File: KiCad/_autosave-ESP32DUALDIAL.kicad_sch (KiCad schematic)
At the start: 84 parts, among them J1 SERVICE, J2 Conn_01x04_Male, J3 mode, J5 Conn_01x03_Male, J6 Conn_01x02_Male, J7 Conn_01x02_Male, J8 Conn_01x02_Male, M1 Fan_CPU_4pin, M2 Fan_CPU_4pin, Q1 Q_NMOS_GDS, SW1 Rotary_Encoder_Switch, SW2 Rotary_Encoder_Switch, U1 CR2013-MI2120, U10 Mini560_DC-DC_JW5068A, U2 ESP-WROOM-32, U3 QS-1205CME-3A_MINIDC-DC_12-24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, U4 DHT11, U5 S108T02, U6 S108T02, U7 S108T02, U8 S108T02, U9 TBD62783A

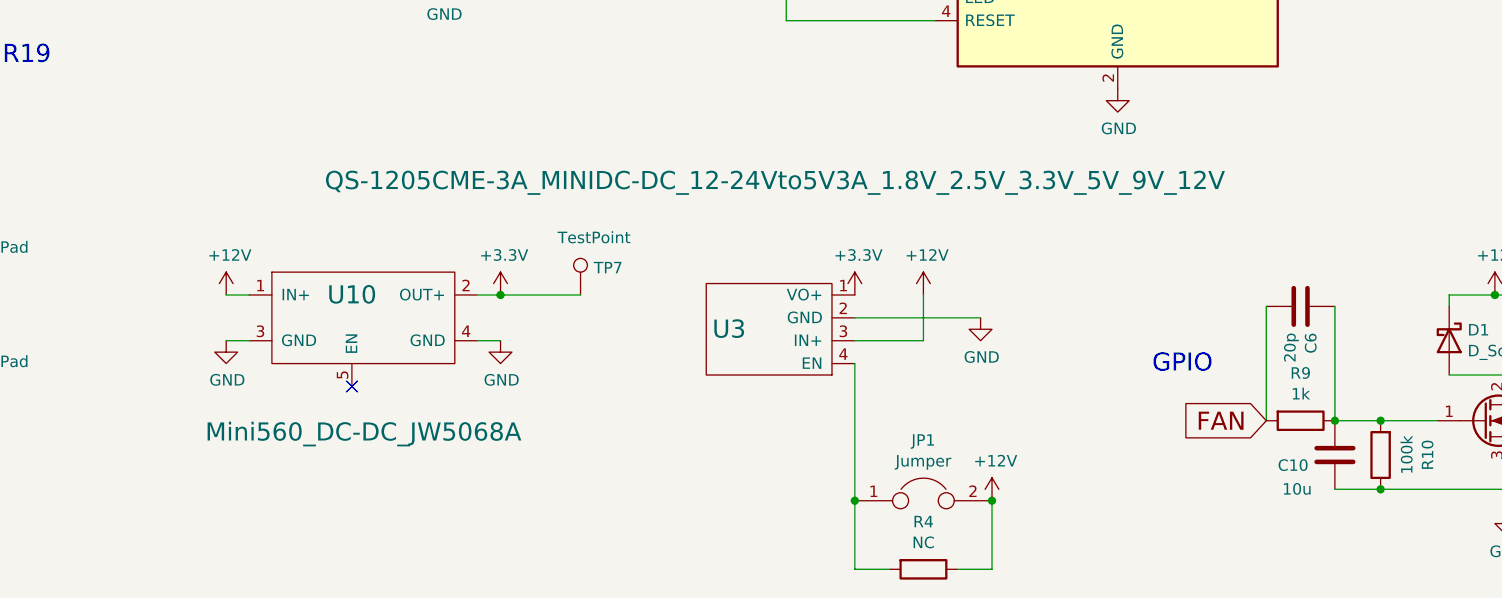
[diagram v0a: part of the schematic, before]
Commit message: v8
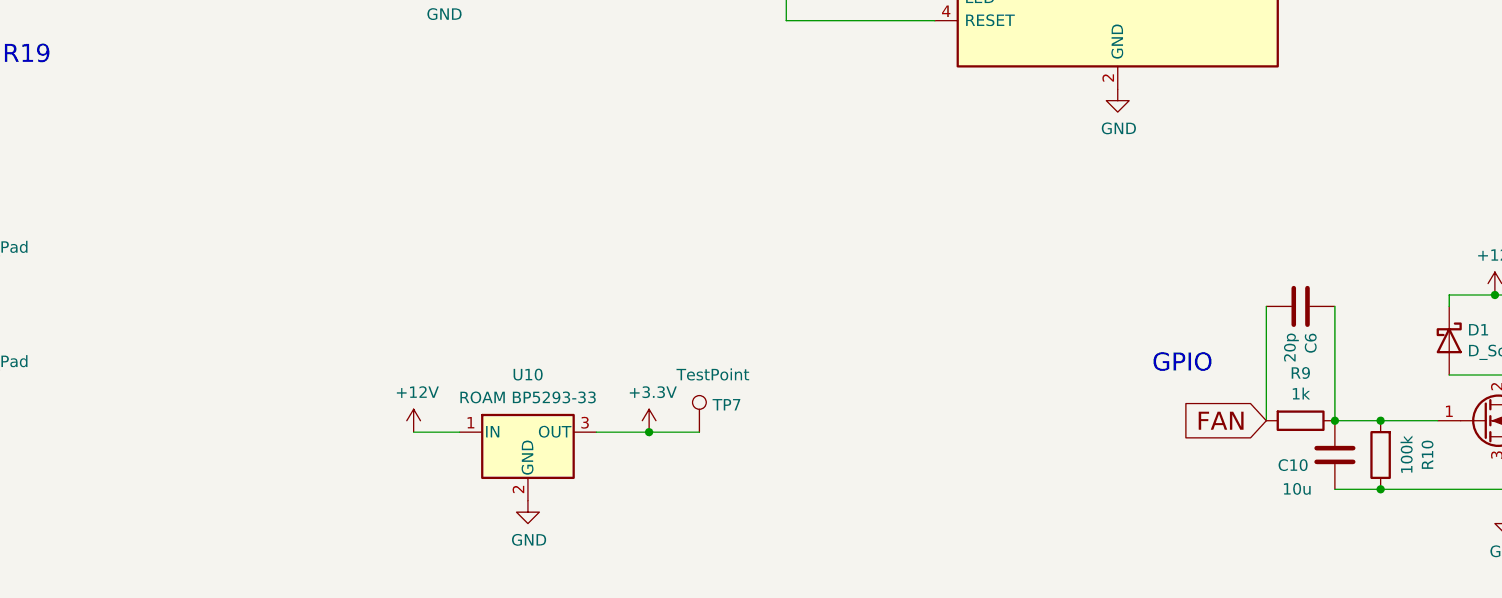
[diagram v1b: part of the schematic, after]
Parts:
- removed JP1: Jumper, Jumper:SolderJumper-2_P1.3mm_Bridged_Pad1.0x1.5mm, symbol ESP32DUALDIAL-rescue:Jumper-Device
- removed R4: NC, Resistor_SMD:R_0603_1608Metric, symbol Device:R
- removed U10: Mini560_DC-DC_JW5068A, library:Mini560_DC-DC_JW5068A, symbol ESP32DUALDIAL-rescue:Mini560_DC-DC_JW5068A-nanbuwks
- removed U3: QS-1205CME-3A_MINIDC-DC_12-24Vto5V3A_1.8V_2.5V_3.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, library:QS-1205CME-3A_MINIDC-DC_12-24Vto5V3A_1.8V_2.5V_3.3V_5V_9V_12V, symbol ESP32DUALDIAL-rescue:QS-1205CME-3A_MINIDC-DC_12-24Vto5V3A_1.8V_2.5V_3.3V_5V_9V_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
- added U10: ROAM BP5293-33, Converter_DCDC:Converter_DCDC_RECOM_R-78E-0.5_THT, symbol Regulator_Switching:R-78E3.3-1.0
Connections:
- net +12V: now also U10.1 (IN)
- net +3V3: now also U10.3 (OUT)
- net Earth: now also U10.2 (GND)
- no-connect marks 26 -> 25
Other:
- moved on the sheet: TP7
